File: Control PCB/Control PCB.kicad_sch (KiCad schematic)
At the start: 27 parts, among them J1 L_Motor_XT30_F, J2 R_Motor_XT30_F, J3 Motor_Power_XT30_M, J4 Sense_L, J5 Sense_R, J6 Amp_power_XT30_M, Q1 IRLZ44N, Q2 IRLZ44N, U1 TL071, U2 TL071

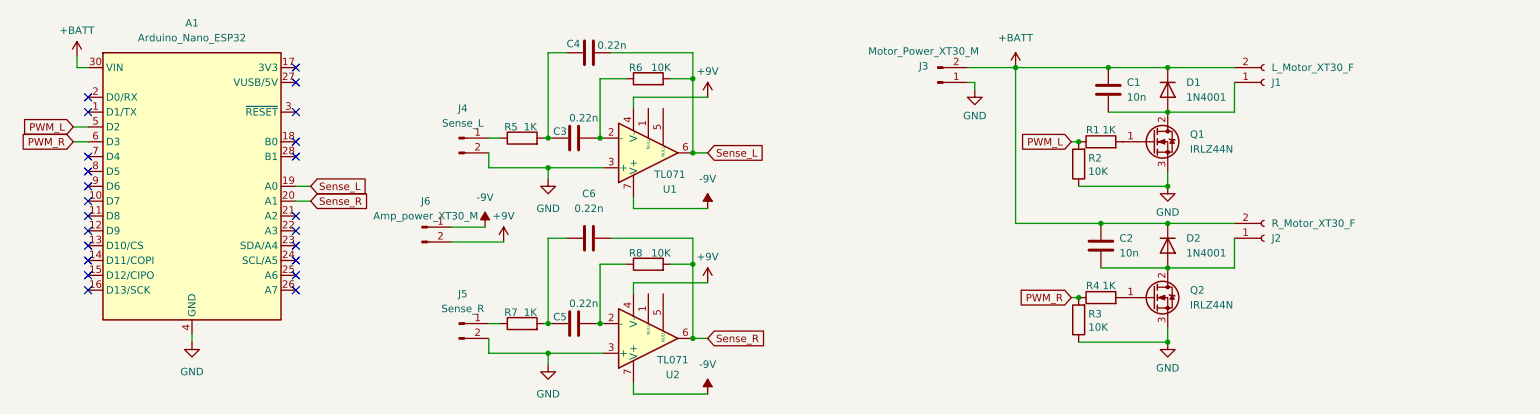
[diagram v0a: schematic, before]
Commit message: Add files via upload
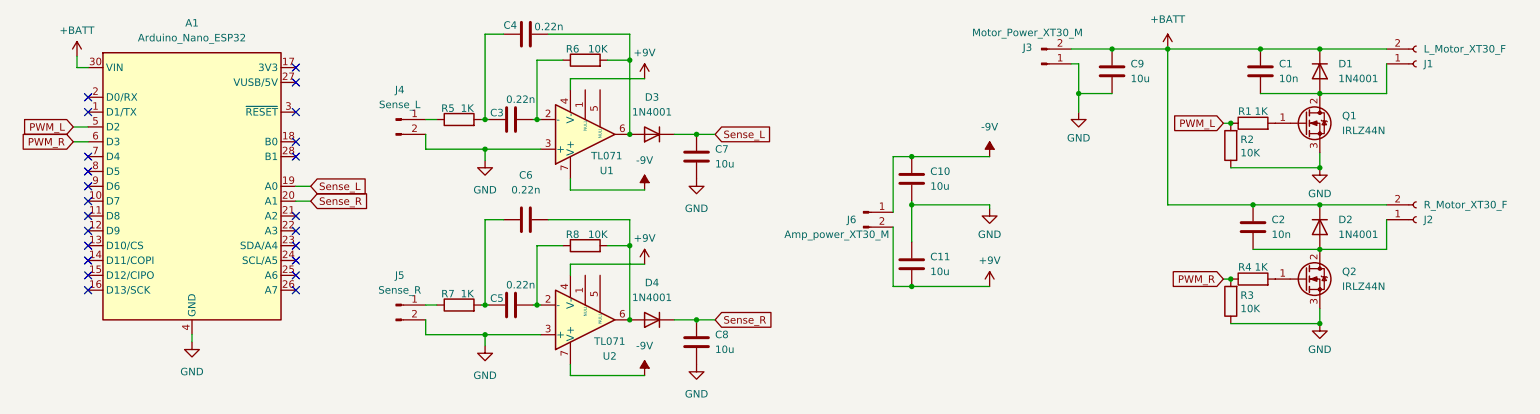
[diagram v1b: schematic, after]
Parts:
- added C10, C11, C7, C8, C9: 10u, Capacitor_THT:C_Rect_L4.6mm_W2.0mm_P2.50mm_MKS02_FKP02, symbol Device:C
- added D3, D4: 1N4001, Diode_THT:D_DO-41_SOD81_P10.16mm_Horizontal, symbol Diode:1N4001
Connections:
- net +9V: now also C11.2
- net +BATT: now also C9.1
- net -9V: now also C10.1
- net GND: now also C10.2, C11.1, C7.2, C8.2, C9.2
- net Sense_L: now also C7.1, D3.1 (K); no longer C4.2, R6.2, U1.6
- net Sense_R: now also C8.1, D4.1 (K); no longer C6.1, R8.2, U2.6
- new net: C6.1, D4.2 (A), R8.2, U2.6
- new net: C4.2, D3.2 (A), R6.2, U1.6
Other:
- moved on the sheet: C1, C2, C3, C4, C5, C6, D1, D2, J1, J2, J3, J4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
